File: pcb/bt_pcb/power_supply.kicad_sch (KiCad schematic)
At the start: 23 parts, among them IC1 LTC3621EMS8E-25#PBF, J17 Conn_01x01, J6 Jack-DC, U1 TLV76133DCY, U2 TLV76133DCY

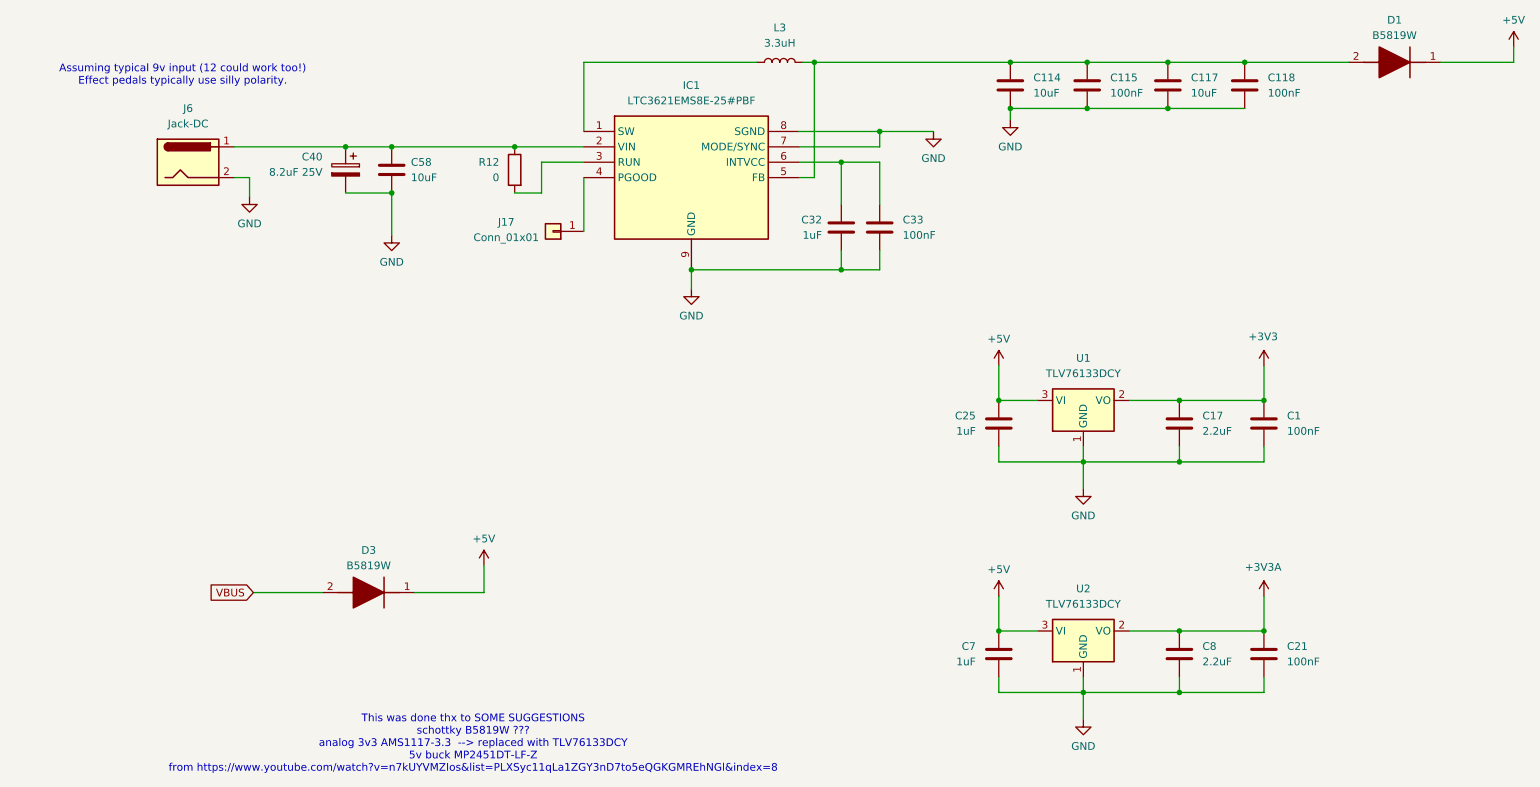
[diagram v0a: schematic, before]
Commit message: solving some erc warnings and errors
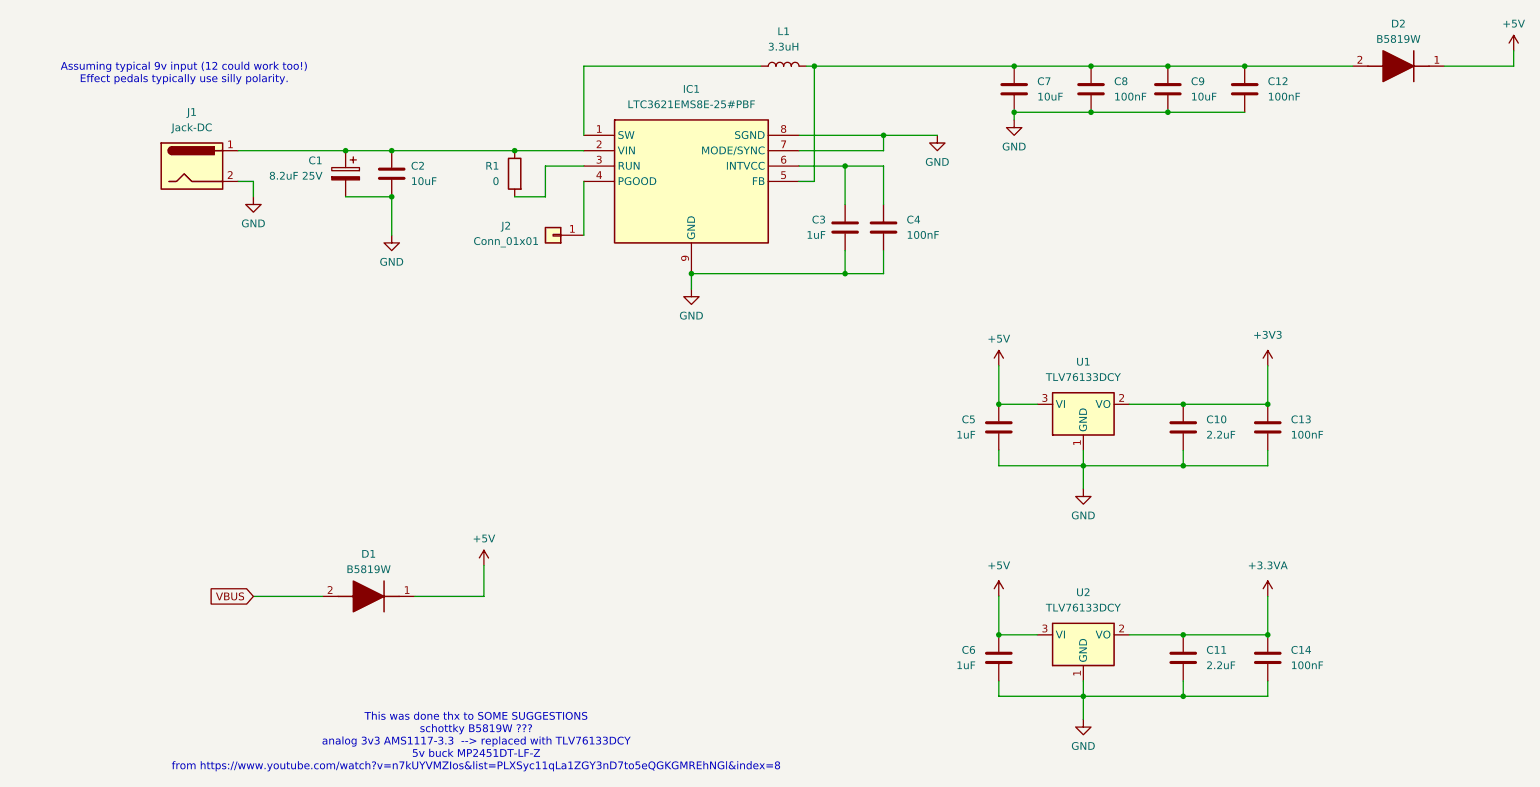
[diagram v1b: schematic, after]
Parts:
- renumbered C40 to C1, C17 to C10, C8 to C11, C118 to C12, C1 to C13, C21 to C14, C58 to C2, C32 to C3, C33 to C4, C25 to C5, C7 to C6, C114 to C7, C115 to C8, C117 to C9, D3 to D1, D1 to D2, J6 to J1, J17 to J2, L3 to L1, R12 to R1
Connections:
- net +3V3A renamed +3.3VA
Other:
- moved on the sheet: C1, C10, C11, C12, C13, C14, C2, C3, C4, C5, C6, C7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
